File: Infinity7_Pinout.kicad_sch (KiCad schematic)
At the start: 4 parts

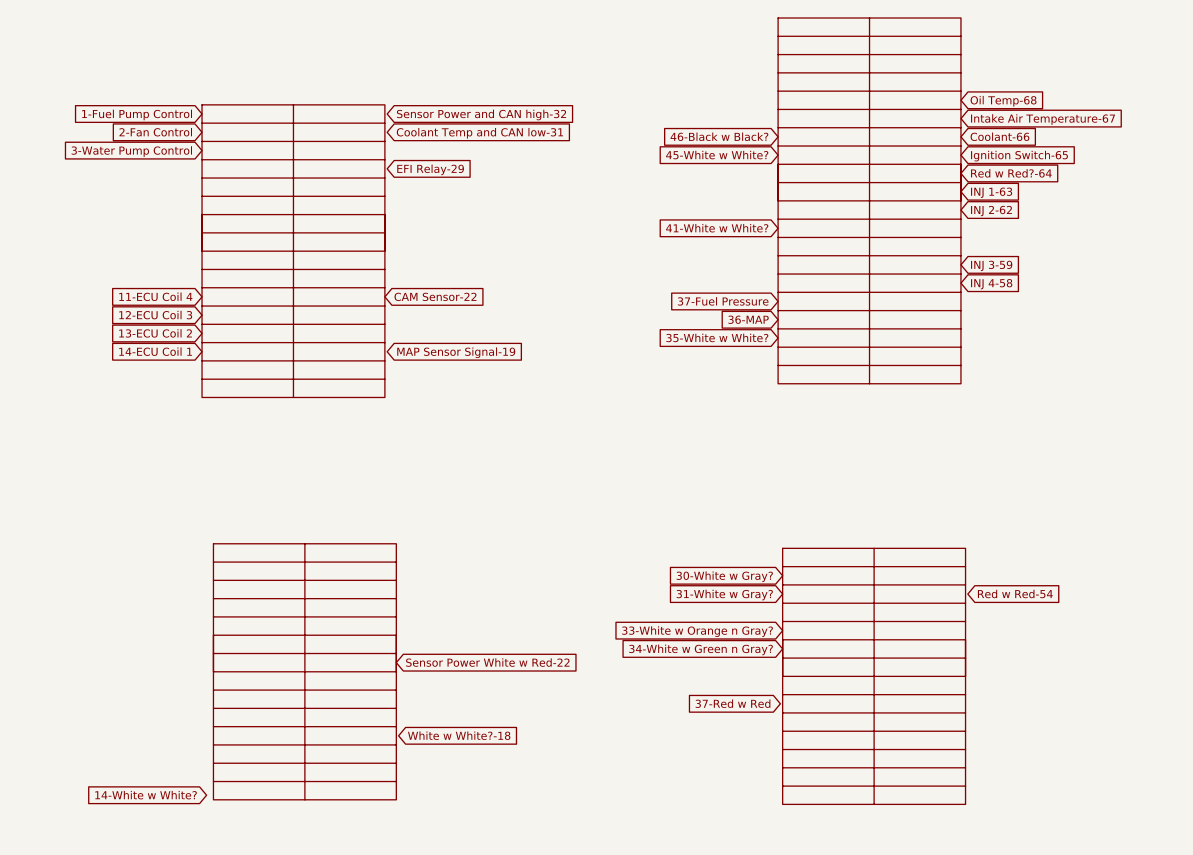
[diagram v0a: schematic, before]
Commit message: Connector Numbers 1
Added Numbers to all of the connectors that were numbered and in KiCad so far
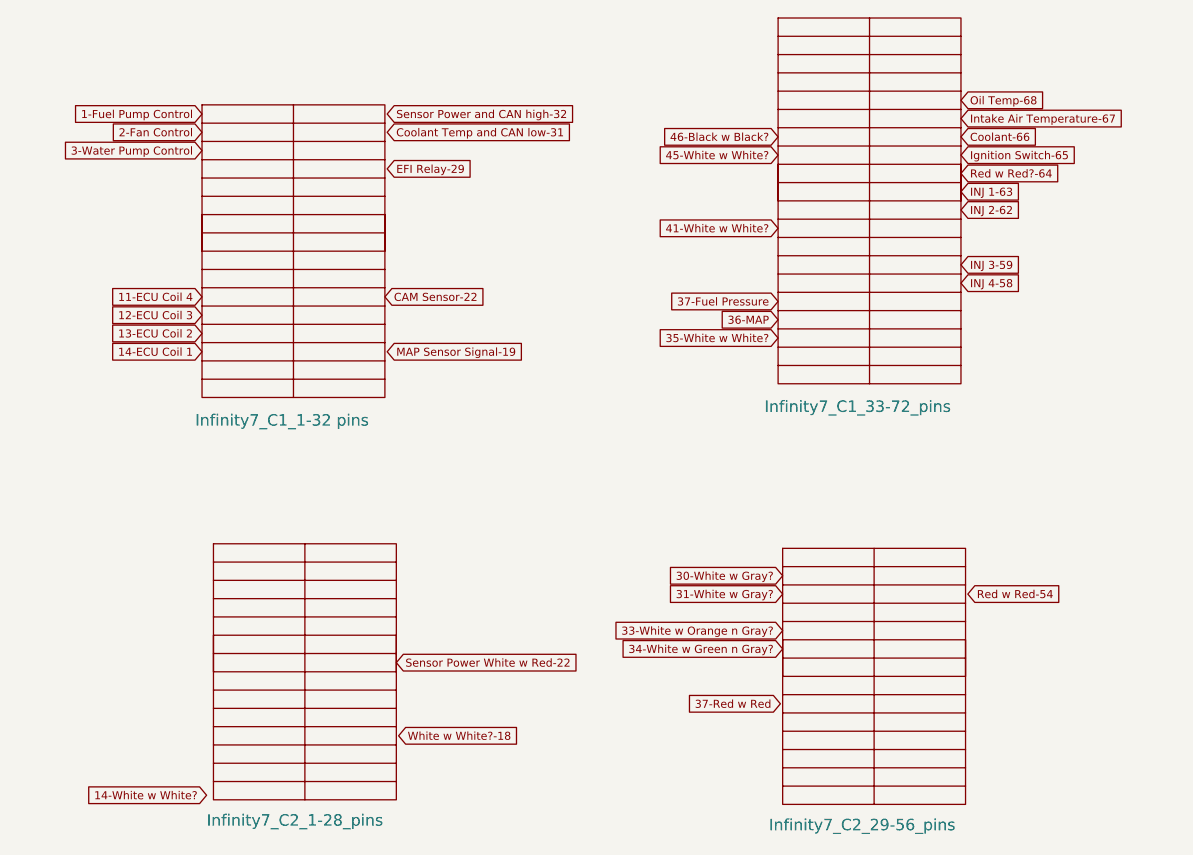
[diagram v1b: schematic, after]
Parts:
- U?: value (none) -> Infinity7_C2_29-56_pins
- U?: value (none) -> Infinity7_C1_33-72_pins
- U?: value (none) -> Infinity7_C2_1-28_pins
- U?: value (none) -> Infinity7_C1_1-32 pins
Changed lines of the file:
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@@
       (effects (font (size 1.27 1.27)) hide)
     )
-    (property "Value" "" (id 1) (at 169.164 130.048 0)
+    (property "Value" "Infinity7_C2_29-56_pins" (id 1) (at 169.164 130.048 0)
       (effects (font (size 1.27 1.27)) (justify left))
     )
@@
       (effects (font (size 1.27 1.27)) hide)
     )
-    (property "Value" "" (id 1) (at 168.656 83.566 0)
+    (property "Value" "Infinity7_C1_33-72_pins" (id 1) (at 168.656 83.566 0)
       (effects (font (size 1.27 1.27)) (justify left))
     )
@@
       (effects (font (size 1.27 1.27)) hide)
     )
-    (property "Value" "" (id 1) (at 106.68 129.54 0)
+    (property "Value" "Infinity7_C2_1-28_pins" (id 1) (at 106.68 129.54 0)
       (effects (font (size 1.27 1.27)) (justify left))
     )
@@
       (effects (font (size 1.27 1.27)) hide)
     )
-    (property "Value" "" (id 1) (at 105.41 85.09 0)
+    (property "Value" "Infinity7_C1_1-32 pins" (id 1) (at 105.41 85.09 0)
       (effects (font (size 1.27 1.27)) (justify left))
     )

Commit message: Updated Connectors
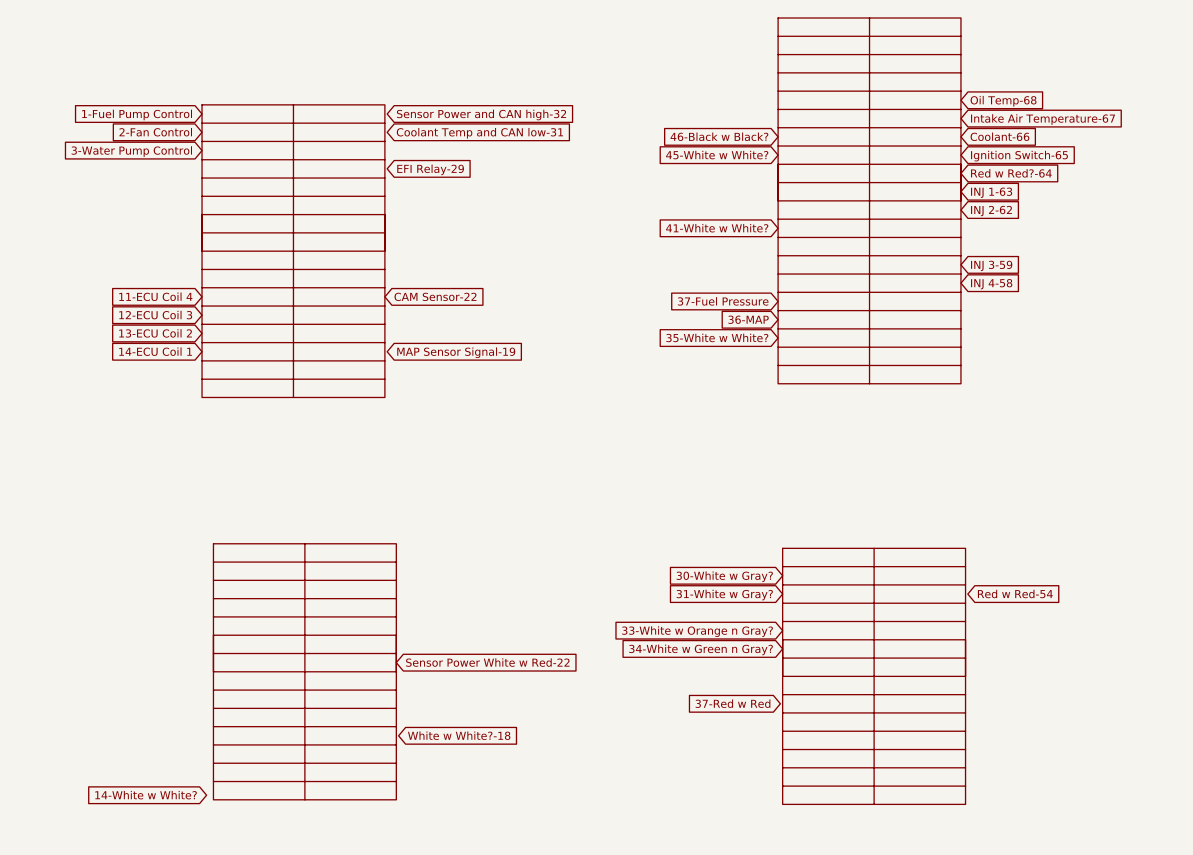
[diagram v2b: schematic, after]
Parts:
- U?: value Infinity7_C2_29-56_pins -> (none)
- U?: value Infinity7_C1_33-72_pins -> (none)
- U?: value Infinity7_C2_1-28_pins -> (none)
- U?: value Infinity7_C1_1-32 pins -> (none)
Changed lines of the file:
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@@
       (effects (font (size 1.27 1.27)) hide)
     )
-    (property "Value" "Infinity7_C2_29-56_pins" (id 1) (at 169.164 130.048 0)
+    (property "Value" "" (id 1) (at 169.164 130.048 0)
       (effects (font (size 1.27 1.27)) (justify left))
     )
@@
       (effects (font (size 1.27 1.27)) hide)
     )
-    (property "Value" "Infinity7_C1_33-72_pins" (id 1) (at 168.656 83.566 0)
+    (property "Value" "" (id 1) (at 168.656 83.566 0)
       (effects (font (size 1.27 1.27)) (justify left))
     )
@@
       (effects (font (size 1.27 1.27)) hide)
     )
-    (property "Value" "Infinity7_C2_1-28_pins" (id 1) (at 106.68 129.54 0)
+    (property "Value" "" (id 1) (at 106.68 129.54 0)
       (effects (font (size 1.27 1.27)) (justify left))
     )
@@
       (effects (font (size 1.27 1.27)) hide)
     )
-    (property "Value" "Infinity7_C1_1-32 pins" (id 1) (at 105.41 85.09 0)
+    (property "Value" "" (id 1) (at 105.41 85.09 0)
       (effects (font (size 1.27 1.27)) (justify left))
     )
